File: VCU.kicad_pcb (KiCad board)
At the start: 2 copper layers, 45.6 x 40.3 mm, 48 parts, among them J1 Conn_02x03_Top_Bottom, J2 2x3_Conn, J4 UJ20-C-H-G-SMT-4-P16-TR, J5 Conn_01x02, SW2 SW_Push, U1 ESP32-S3-WROOM-1, U3 SN65HVD230, U4 USBLC6-2SC6, U5 MCP2518FD-xQBB, U6 MCP6001-OT, U7 PTCAN3413DR, U8 AP2112K-3.3, Y1 40Mhz Crystal

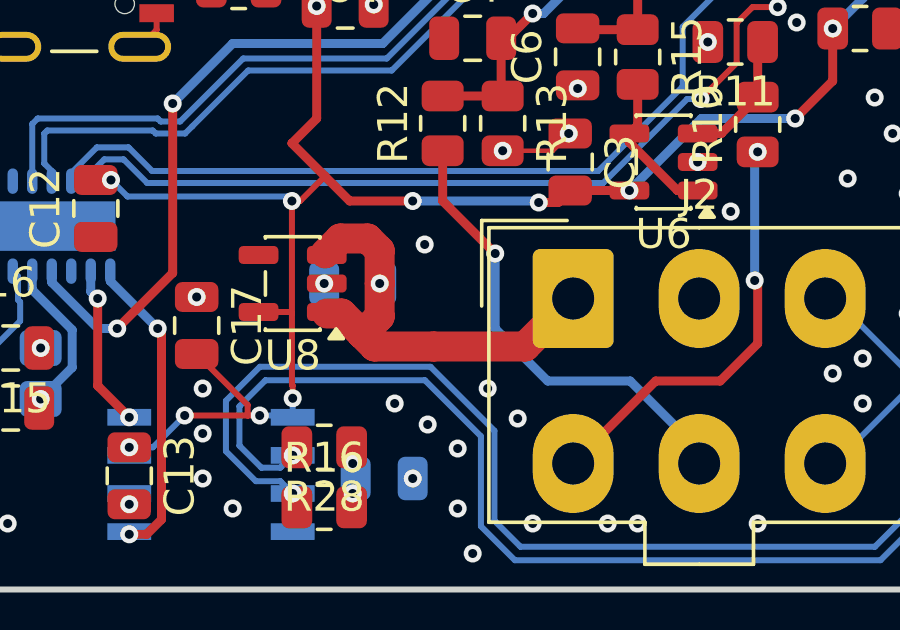
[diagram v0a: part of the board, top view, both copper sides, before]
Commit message: lol
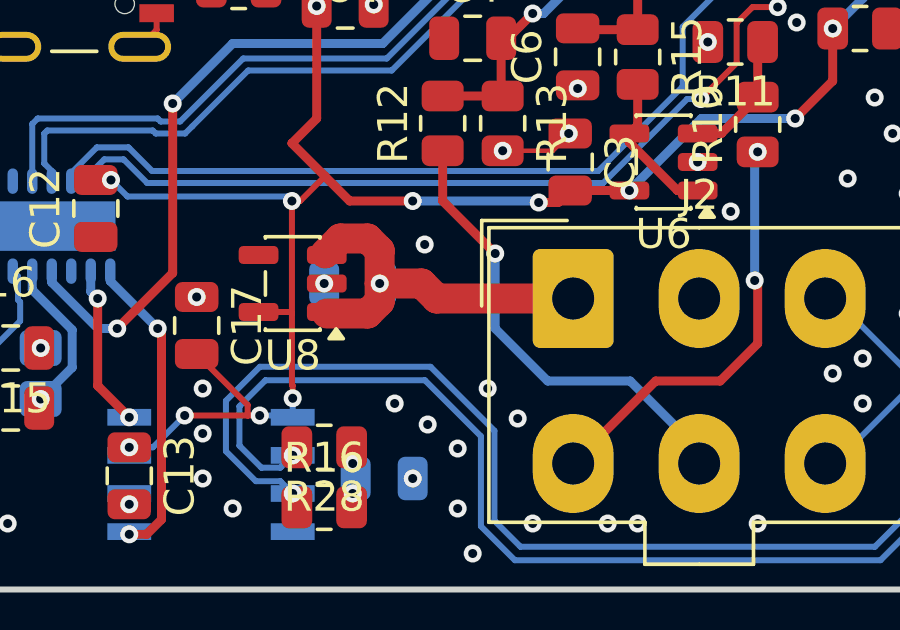
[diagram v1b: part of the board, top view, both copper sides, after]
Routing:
- net Vin(5V): track 14.5 -> 12.5 mm
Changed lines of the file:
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@@
 	)
 	(segment
-		(start 81.315 73.685)
-		(end 80.63 73)
+		(start 81.9 72.6)
+		(end 81.9 72)
 		(width 1)
 		(layer "F.Cu")
@@
 	)
 	(segment
-		(start 83.7 74.1)
-		(end 81.73 74.1)
-		(width 1)
-		(layer "F.Cu")
-		(net "Vin(5V)")
-	)
-	(segment
-		(start 86.75 74.1)
-		(end 83.7 74.1)
+		(start 81.9 72)
+		(end 83.3 72)
 		(width 1)
 		(layer "F.Cu")
@@
 	)
 	(segment
-		(start 81.315 73.685)
-		(end 81.9 73.1)
+		(start 83.3 72)
+		(end 83.8 72.5)
 		(width 1)
 		(layer "F.Cu")
@@
 	)
 	(segment
-		(start 81.9 73.1)
-		(end 81.9 72)
+		(start 81.5 73)
+		(end 81.9 72.6)
 		(width 1)
 		(layer "F.Cu")
@@
 	)
 	(segment
-		(start 80.63 73)
-		(end 80.1375 73)
+		(start 83.8 72.5)
+		(end 88.35 72.5)
 		(width 1)
 		(layer "F.Cu")
@@
 	)
 	(segment
-		(start 81.73 74.1)
-		(end 81.315 73.685)
+		(start 80.1375 73)
+		(end 81.5 73)
 		(width 1)
 		(layer "F.Cu")
-		(net "Vin(5V)")
-	)
-	(segment
-		(start 88.35 72.5)
-		(end 86.75 74.1)
-		(width 1)
-		(layer "F.Cu")
